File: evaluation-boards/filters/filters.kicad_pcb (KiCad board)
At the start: 4 copper layers, 15 x 145 mm, 28 parts, among them J1 CONN_COAXIAL, J10 CONN_COAXIAL, J11 CONN_COAXIAL, J12 CONN_COAXIAL, J13 CONN_COAXIAL, J14 CONN_COAXIAL, J15 CONN_COAXIAL, J16 CONN_COAXIAL, J17 CONN_COAXIAL, J18 CONN_COAXIAL, J19 CONN_COAXIAL, J2 CONN_COAXIAL, J20 CONN_COAXIAL, J3 CONN_COAXIAL, J4 CONN_COAXIAL, J5 CONN_COAXIAL, J6 CONN_COAXIAL, J7 CONN_COAXIAL, J8 CONN_COAXIAL, J9 CONN_COAXIAL, U1 FIL-DEA, U2 FIL-DEA, U3 FIL-LP0603, U4 FIL-LP0603, U5 5130BP18U4060, U6 DEA202484HT, U7 2450HP

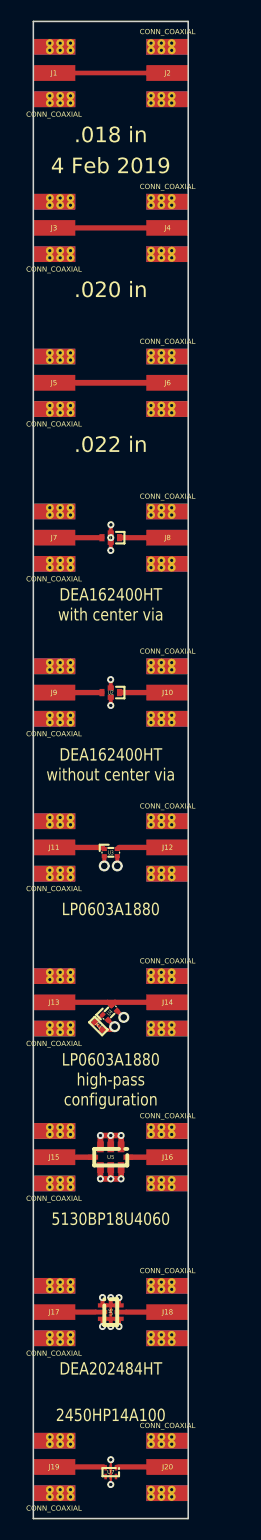
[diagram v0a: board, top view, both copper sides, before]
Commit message: Update filter test board
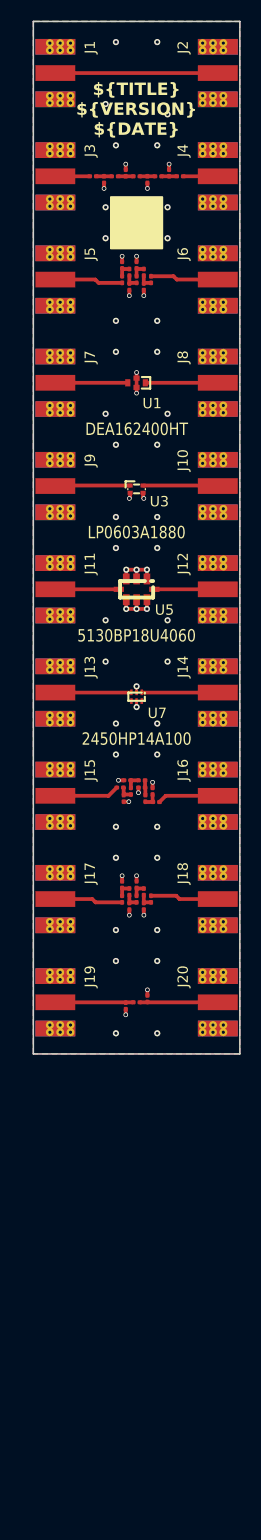
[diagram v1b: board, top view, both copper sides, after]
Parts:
- removed the J10 at (155.0, 95.0)
- removed the J13 at (140.0, 125.0)
- removed the J14 at (155.0, 125.0)
- removed the J9 at (140.0, 95.0)
- removed U2: FIL-DEA, gsg-modules:FIL-DEA-0603
- removed U4: FIL-LP0603, gsg-modules:LP0603
- removed U6: DEA202484HT, gsg-modules:DEA202484HT
- added C1: C, Capacitor_SMD:C_0201_0603Metric, F.Cu at (145.8, 45.0)
- added C10: C, Capacitor_SMD:C_0201_0603Metric, F.Cu at (151.4, 55.0)
- added C11: C, Capacitor_SMD:C_0201_0603Metric, F.Cu at (148.4, 104.2)
- added C12: C, Capacitor_SMD:C_0201_0603Metric, F.Cu at (149.4, 104.5)
- added C13: C, Capacitor_SMD:C_0201_0603Metric, F.Cu at (150.5, 103.5)
- added C14: C, Capacitor_SMD:C_0201_0603Metric, F.Cu at (150.8, 105.2)
- added C15: C, Capacitor_SMD:C_0201_0603Metric, F.Cu at (151.9, 105.6)
- added C16: C, Capacitor_SMD:C_0201_0603Metric, F.Cu at (148.6, 115.0)
- added C17: C, Capacitor_SMD:C_0201_0603Metric, F.Cu at (149.3, 114.3)
- added C18: C, Capacitor_SMD:C_0201_0603Metric, F.Cu at (150.0, 115.0)
- added C19: C, Capacitor_SMD:C_0201_0603Metric, F.Cu at (150.7, 114.3)
- added C2: C, Capacitor_SMD:C_0201_0603Metric, F.Cu at (147.9, 45.0)
- added C20: C, Capacitor_SMD:C_0201_0603Metric, F.Cu at (151.4, 115.0)
- added C3: C, Capacitor_SMD:C_0201_0603Metric, F.Cu at (150.0, 45.0)
- added C4: C, Capacitor_SMD:C_0201_0603Metric, F.Cu at (152.1, 45.0)
- added C5: C, Capacitor_SMD:C_0201_0603Metric, F.Cu at (154.2, 45.0)
- added C6: C, Capacitor_SMD:C_0201_0603Metric, F.Cu at (148.6, 55.0)
- added C7: C, Capacitor_SMD:C_0201_0603Metric, F.Cu at (149.3, 54.3)
- added C8: C, Capacitor_SMD:C_0201_0603Metric, F.Cu at (150.0, 55.0)
- added C9: C, Capacitor_SMD:C_0201_0603Metric, F.Cu at (150.7, 54.3)
- added J15: Conn_Coaxial, sma-variants:Linx_SMA_CONSMA003.062, F.Cu at (140.0, 105.0)
- added J16: Conn_Coaxial, sma-variants:Linx_SMA_CONSMA003.062, F.Cu at (160.0, 105.0)
- added J19: Conn_Coaxial, sma-variants:Linx_SMA_CONSMA003.062, F.Cu at (140.0, 125.0)
- added J20: Conn_Coaxial, sma-variants:Linx_SMA_CONSMA003.062, F.Cu at (160.0, 125.0)
- added L1: L, Inductor_SMD:L_0201_0603Metric, F.Cu at (146.8, 45.3)
- added L10: L, Inductor_SMD:L_0201_0603Metric, F.Cu at (149.1, 103.5)
- added L11: L, Inductor_SMD:L_0201_0603Metric, F.Cu at (150.5, 104.2)
- added L12: L, Inductor_SMD:L_0201_0603Metric, F.Cu at (151.6, 104.5)
- added L13: L, Inductor_SMD:L_0201_0603Metric, F.Cu at (148.6, 113.6)
- added L14: L, Inductor_SMD:L_0201_0603Metric, F.Cu at (149.3, 115.7)
- added L15: L, Inductor_SMD:L_0201_0603Metric, F.Cu at (150.0, 113.6)
- added L16: L, Inductor_SMD:L_0201_0603Metric, F.Cu at (150.7, 115.7)
- added L2: L, Inductor_SMD:L_0201_0603Metric, F.Cu at (148.9, 44.7)
- added L3: L, Inductor_SMD:L_0201_0603Metric, F.Cu at (151.1, 45.3)
- added L4: L, Inductor_SMD:L_0201_0603Metric, F.Cu at (153.2, 44.7)
- added L5: L, Inductor_SMD:L_0201_0603Metric, F.Cu at (148.6, 53.6)
- added L6: L, Inductor_SMD:L_0201_0603Metric, F.Cu at (149.3, 55.7)
- added L7: L, Inductor_SMD:L_0201_0603Metric, F.Cu at (150.0, 53.6)
- added L8: L, Inductor_SMD:L_0201_0603Metric, F.Cu at (150.7, 55.7)
- added L9: L, Inductor_SMD:L_0201_0603Metric, F.Cu at (148.8, 105.2)
- added R2: R, Resistor_SMD:R_0201_0603Metric, F.Cu at (150.0, 125.0)
- added R3: R, Resistor_SMD:R_0201_0603Metric, F.Cu at (151.1, 124.7)
- J1, J17, J18, J2, J3, J4, J5, J6, J7, J8: value CONN_COAXIAL -> Conn_Coaxial; footprint gsg-modules:SMA-EDGE -> sma-variants:Linx_SMA_CONSMA003.062
- J10: renamed from J12; value CONN_COAXIAL -> Conn_Coaxial; footprint gsg-modules:SMA-EDGE -> sma-variants:Linx_SMA_CONSMA003.062
- J11: renamed from J15; value CONN_COAXIAL -> Conn_Coaxial; footprint gsg-modules:SMA-EDGE -> sma-variants:Linx_SMA_CONSMA003.062
- J12: renamed from J16; value CONN_COAXIAL -> Conn_Coaxial; footprint gsg-modules:SMA-EDGE -> sma-variants:Linx_SMA_CONSMA003.062
- J13: renamed from J19; value CONN_COAXIAL -> Conn_Coaxial; footprint gsg-modules:SMA-EDGE -> sma-variants:Linx_SMA_CONSMA003.062
- J14: renamed from J20; value CONN_COAXIAL -> Conn_Coaxial; footprint gsg-modules:SMA-EDGE -> sma-variants:Linx_SMA_CONSMA003.062
- J9: renamed from J11; value CONN_COAXIAL -> Conn_Coaxial; footprint gsg-modules:SMA-EDGE -> sma-variants:Linx_SMA_CONSMA003.062
- R1: value 0 -> R; footprint gsg-modules:0402 -> Resistor_SMD:R_0201_0603Metric
- U5: value 5130BP18U4060 -> VAL**
- moved J14 75.2 mm to (160.0, 95.0)
- moved U7 75.1 mm to (150.0, 95.4)
- moved J13 75.0 mm to (140.0, 95.0)
- moved J12 55.2 mm to (160.0, 85.0)
- moved U5 55.1 mm to (150.0, 85.0)
- moved J11 55.0 mm to (140.0, 85.0)
- moved J18 40.3 mm to (160.0, 115.0)
- moved J17 40.0 mm to (140.0, 115.0)
- moved J10 35.4 mm to (160.0, 75.0)
- moved U3 35.3 mm to (150.0, 75.3)
- moved J9 35.0 mm to (140.0, 75.0)
- moved J8 15.8 mm to (160.0, 65.0)
- moved U1 15.2 mm to (150.0, 65.0)
- moved J7 15.0 mm to (140.0, 65.0)
- moved J6 11.2 mm to (160.0, 55.0)
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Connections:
- J3 pad 1: Net-(J3-Pad1) -> Net-(J3-In)
- J4 pad 1: Net-(J3-Pad1) -> Net-(J4-In)
- J5 pad 1: Net-(J5-Pad1) -> Net-(J5-In)
- J6 pad 1: Net-(J5-Pad1) -> Net-(J6-In)
- R1 pad 2: GND -> Net-(J19-In)
- U7 pad 4: (no net) -> unconnected-(U7-NC-Pad4)
- U7 pad 6: (no net) -> unconnected-(U7-NC-Pad6)
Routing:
- net Net-(J13-Pad1): track 11.9 -> 0.00 mm
- net Net-(J5-Pad1): track 10.9 -> 0.00 mm
- net Net-(J3-Pad1): track 10.9 -> 0.00 mm
- net GND: track 33.3 -> 23.4 mm, vias 23 -> 70
- net Net-(J20-In): track 0.00 -> 7.55 mm
- net Net-(J19-In): track 0.00 -> 7.55 mm
- net Net-(J5-In): track 0.00 -> 6.60 mm
- net Net-(J6-In): track 0.00 -> 6.60 mm
- net Net-(J15-In): track 0.00 -> 6.28 mm
- net Net-(J16-In): track 0.00 -> 5.90 mm
- net Net-(J1-In): track 10.9 -> 15.7 mm
- net Net-(J9-Pad1): track 4.62 -> 0.00 mm
- net Net-(J10-Pad1): track 4.62 -> 0.00 mm
- net Net-(J4-In): track 0.00 -> 3.35 mm
- net Net-(J3-In): track 0.00 -> 3.33 mm
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- added copper zone on B.Cu, net GND
- added copper zone on F.Cu, net GND
- added copper zone on In2.Cu, net GND
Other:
- board size 15 x 145 mm -> 20 x 100 mm
- net class Default removed
- board text added: "${TITLE} ${REVISION} ${ISSUE_DATE}"
- board text added: "DEA162400HT"
- board text removed: ".018 in"
- board text removed: ".020 in"
- board text removed: ".022 in"
- board text removed: "4 Feb 2019"
- board text removed: "DEA162400HT with center via"
- board text removed: "DEA162400HT without center via"
- board text removed: "DEA202484HT"
- board text removed: "LP0603A1880 high-pass configuration"
